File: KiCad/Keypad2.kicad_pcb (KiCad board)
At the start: 2 copper layers, 13.2 x 29 mm, 18 parts, among them J1 Keypad, J2 Prog, U1 SP3485, U2 ESP32-PICO-MINI-02, U3 LMR16006+FB, U4 QR

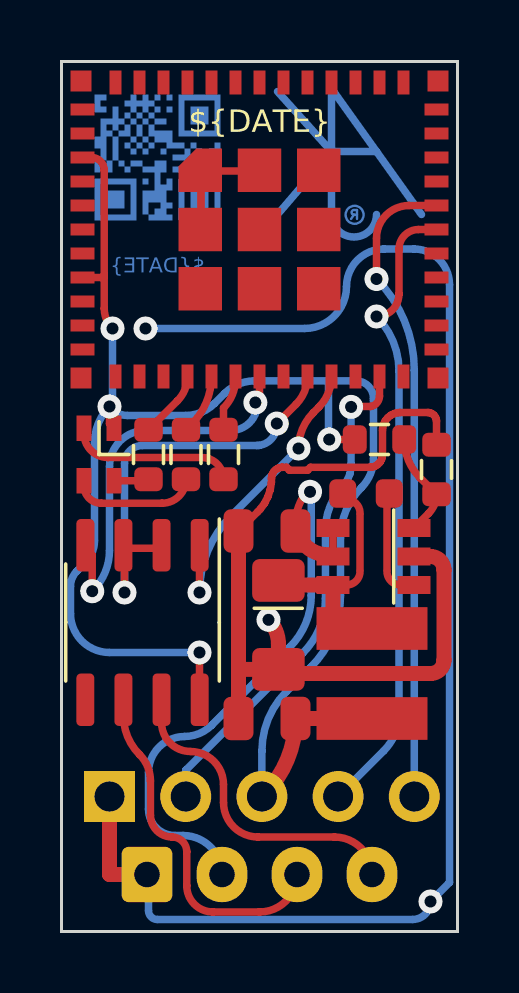
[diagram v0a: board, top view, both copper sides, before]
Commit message: Tweak, getting ready to order
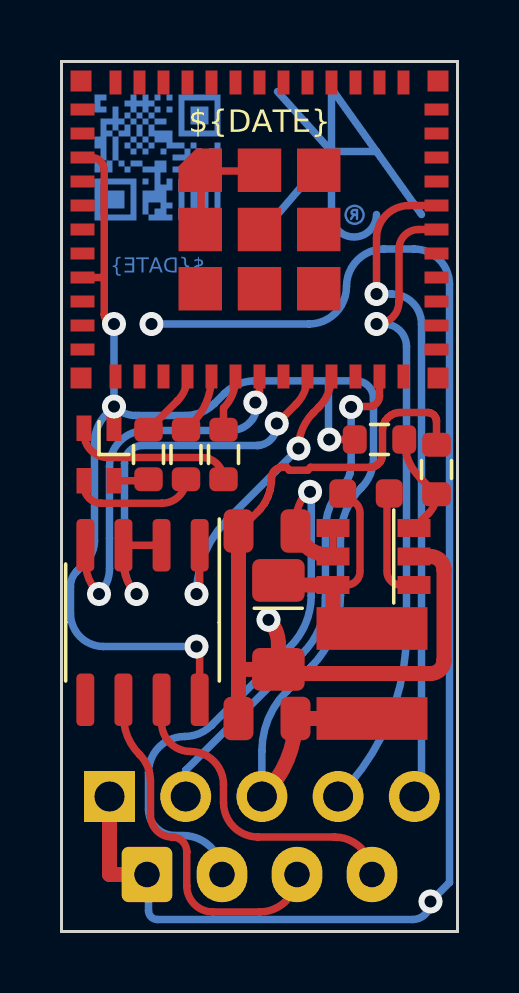
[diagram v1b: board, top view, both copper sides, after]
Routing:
- net O: track 21.5 -> 22.3 mm
